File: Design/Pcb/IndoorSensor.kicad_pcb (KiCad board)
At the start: 2 copper layers, 49.5 x 48.3 mm, 17 parts, among them J1 Conn_01x04_Pin, J2 Conn_01x06_Pin, J3 Conn_01x04_Pin, U1 MH-Z19B, U3 WeMos_D1_mini, U4 module_bme280_alt

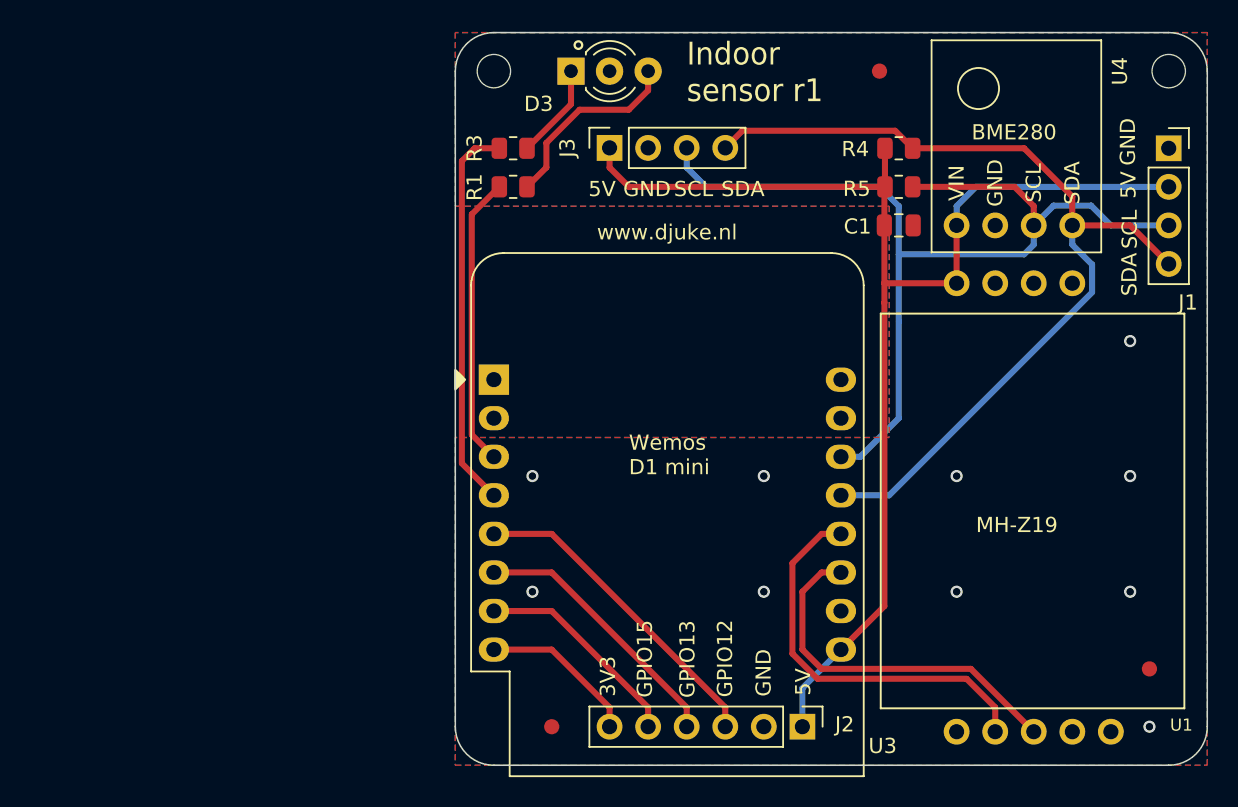
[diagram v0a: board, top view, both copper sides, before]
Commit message: Add revision 2 design
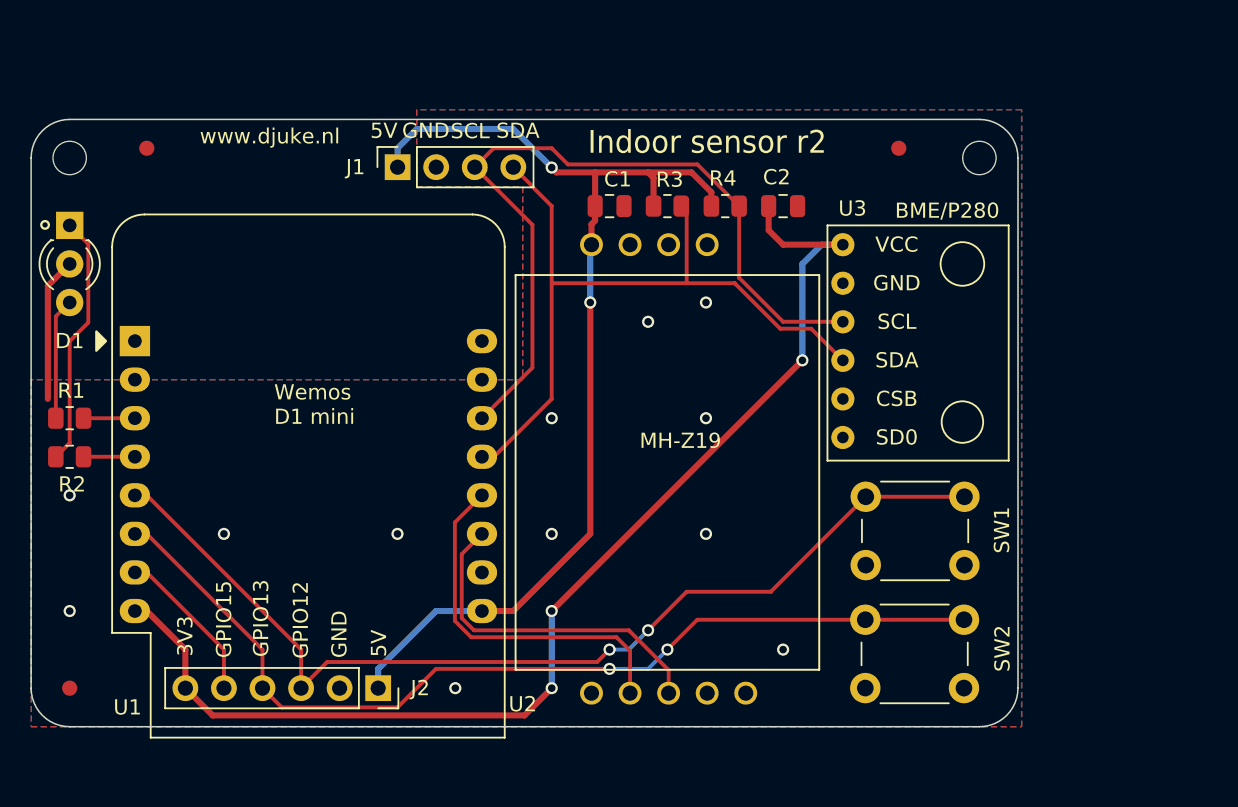
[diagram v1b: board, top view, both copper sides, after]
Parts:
- removed the J1 at (123.2, 86.4)
- removed the R4 at (105.4, 86.4)
- removed U4: module_bme280_alt, Libraries:module_bme280_alt
- added C2: 100n, Capacitor_SMD:C_0805_2012Metric, F.Cu at (97.8, 90.2)
- added R3: 4k7, Resistor_SMD:R_0805_2012Metric, F.Cu at (90.2, 90.2)
- added SW1: SW_Push, Button_Switch_THT:SW_PUSH_6mm_H5mm, F.Cu at (103.2, 109.3)
- added SW2: SW_Push, Button_Switch_THT:SW_PUSH_6mm_H5mm, F.Cu at (103.2, 117.4)
- added U3: module_bme280, Libraries:module_bme280, F.Cu at (106.8, 105.2)
- J2: footprint Connector_PinHeader_2.54mm:PinHeader_1x06_P2.54mm_Vertical -> Connector_PinSocket_2.54mm:PinSocket_1x06_P2.54mm_Vertical
- U1: renamed from U3; footprint Module:WEMOS_D1_mini_light -> RF_Module:WEMOS_D1_mini_light
- U2: renamed from U1; footprint MH-Z19B:MH-Z19B-FOOT -> Libraries:MH-Z19B-FOOT
- moved FID3 74.4 mm to (55.9, 86.4)
- moved R2 35.6 mm to (50.8, 106.7), turned to 180 degrees
- moved D1 34.5 mm to (50.8, 91.4), turned to -90 degrees
- moved R1 32.9 mm to (50.8, 104.1), turned to 180 degrees
- moved FID1 31.9 mm to (50.8, 121.9)
- moved H2 28.5 mm to (50.8, 87.0)
- moved J2 28.1 mm to (71.1, 121.9)
- moved U2 24.2 mm to (85.2, 92.7)
- moved U1 23.8 mm to (55.1, 99.1)
- moved C1 19.1 mm to (86.4, 90.2)
- moved J1 14.0 mm to (72.4, 87.6)
- moved H1 13.7 mm to (110.7, 87.0)
- moved R4 11.5 mm to (94.0, 90.2)
- moved FID2 5.24 mm to (105.4, 86.4)
- renumbered D3 to D1, J3 to J1, R3 to R2, R5 to R4
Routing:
- net +3V3: track 10.5 -> 77.4 mm, vias 0 -> 3
- net GPIO13: track 17.7 -> 63.2 mm, vias 0 -> 2
- net GPIO12: track 21.2 -> 66.6 mm, vias 0 -> 2
- net LED_ERR: track 25.7 -> 3.38 mm
- net LED_OK: track 19.1 -> 3.38 mm
- net +5V: track 84.6 -> 70.7 mm, vias 0 -> 2
- net SCL: track 65.3 -> 51.7 mm
- net SDA: track 61.5 -> 49.0 mm
- net Net-(D1-A1): track 6.28 -> 16.6 mm
- net GND: track 0.00 -> 9.49 mm, vias 10 -> 12
- net Net-(D1-A2): track 12.8 -> 8.00 mm
- net GPIO15: track 14.1 -> 10.5 mm
- net TX: track 26.4 -> 24.2 mm
- net RX: track 24.4 -> 22.7 mm
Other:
- board size 49.5 x 48.3 mm -> 65 x 40 mm
- board text added: "Indoor sensor r2"
- board text removed: "BME280"
- board text removed: "Indoor sensor r1"
